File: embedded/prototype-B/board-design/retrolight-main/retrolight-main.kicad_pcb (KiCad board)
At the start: 2 copper layers, 57 x 19 mm, 31 parts, among them J1 Conn_02x03_Odd_Even, U1 TLC59108xPW

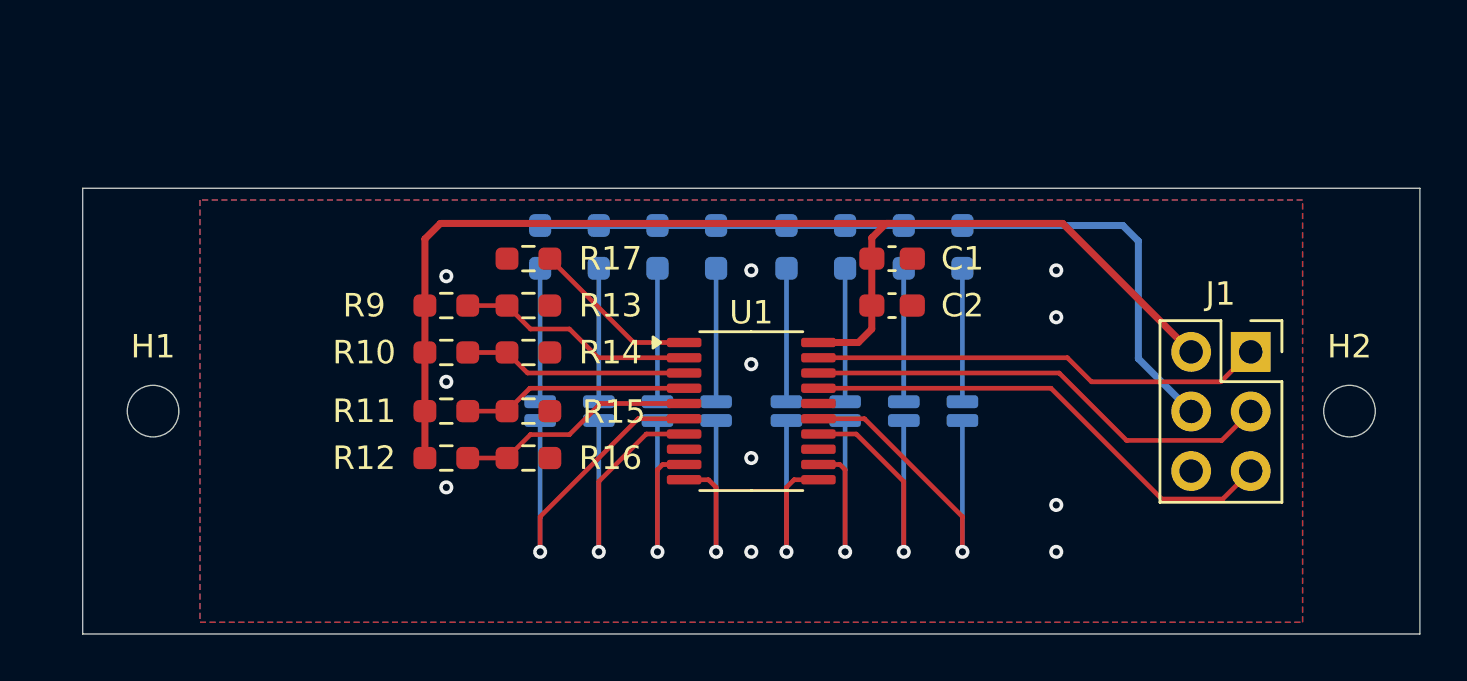
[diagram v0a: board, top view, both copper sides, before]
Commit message: [Light] Rework
Refactored light module design to match the newest changes for the
central unit.

Signed-off-by: Nicolae-Andrei Prodan <vasilenicolaeandrei@gmail.com>
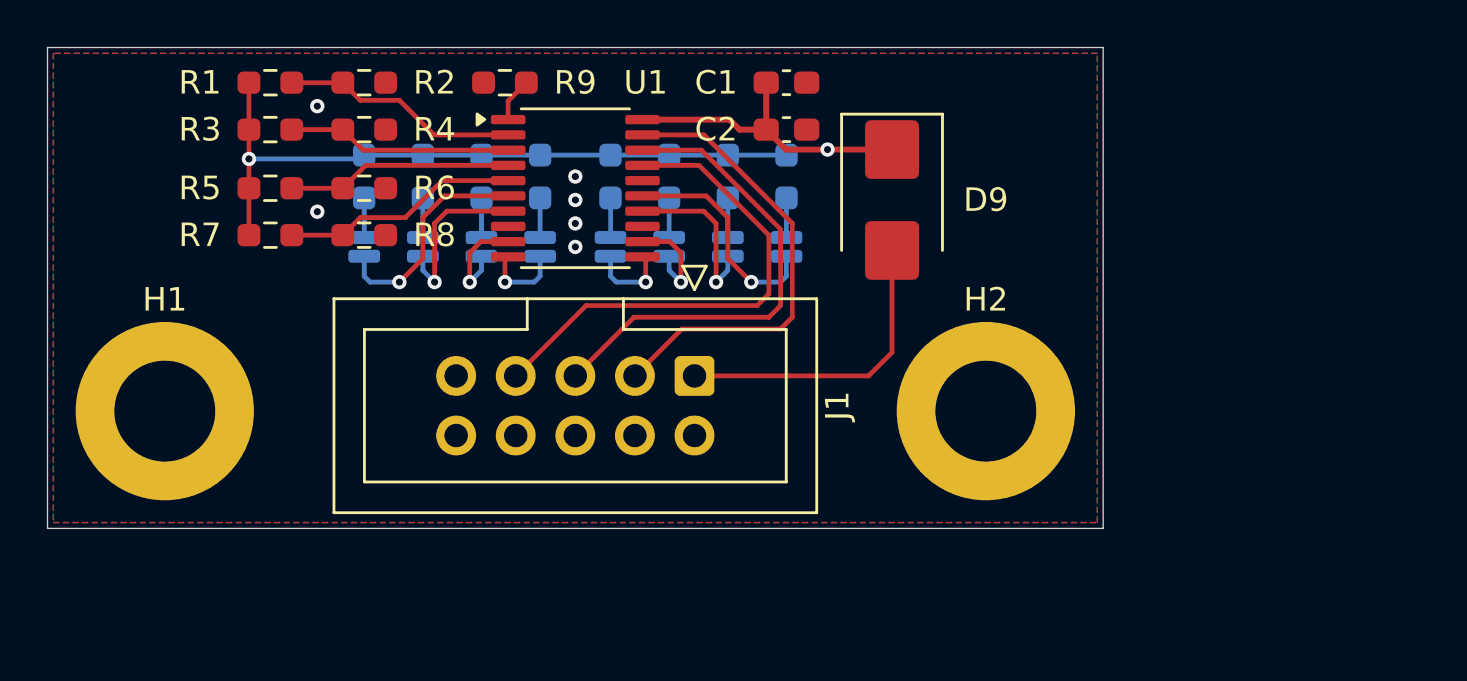
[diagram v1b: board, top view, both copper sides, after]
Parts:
- added D9: MBRS130LT3G, Diode_SMD:D_SMB, F.Cu at (156.0, 91.0)
- H1, H2: value MountingHole -> MountingHole_Pad; footprint MountingHole:MountingHole_2.2mm_M2_ISO7380 -> MountingHole:MountingHole_4.3mm_M4_ISO7380_Pad
- J1: value Conn_02x03_Odd_Even -> Conn_02x05_Odd_Even; footprint Connector_PinSocket_2.54mm:PinSocket_2x03_P2.54mm_Vertical -> Connector_IDC:IDC-Header_2x05_P2.54mm_Vertical
- R1, R3, R5, R7: value 0R/R0603 -> 10K/R0603(NC); moved to F.Cu
- R10, R11, R12: value 10K/R0603(NC) -> 0R/R0603; moved to B.Cu
- R13, R14, R15, R16: moved to B.Cu
- R17: value 375R/R0603 -> 0R/R0603; moved to B.Cu
- R2, R4, R6, R8: moved to F.Cu
- R9: value 10K/R0603(NC) -> 375R/R0603
- moved R7 27.0 mm to (129.5, 92.5), turned to 180 degrees
- moved R8 25.5 mm to (133.5, 92.5), turned to 0 degrees
- moved J1 23.7 mm to (147.6, 98.5), turned to -90 degrees
- moved R5 22.1 mm to (129.5, 90.5), turned to 180 degrees
- moved R6 20.7 mm to (133.5, 90.5), turned to 0 degrees
- moved R3 17.2 mm to (129.5, 88.0), turned to 180 degrees
- moved R4 15.8 mm to (133.5, 88.0), turned to 0 degrees
- moved H2 15.5 mm to (160.0, 100.0)
- moved R16 14.7 mm to (149.0, 90.0), turned to 90 degrees
- moved R1 13.5 mm to (129.5, 86.0), turned to 180 degrees
- moved R2 12.2 mm to (133.5, 86.0), turned to 0 degrees
- moved U1 12.1 mm to (142.5, 90.5)
- moved R12 12.1 mm to (138.5, 90.0), turned to 90 degrees
- moved R15 11.7 mm to (146.5, 90.0), turned to 90 degrees
- moved R17 11.5 mm to (151.5, 90.0), turned to 90 degrees
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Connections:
- J1 pad 1: /SDA -> Net-(D9-A)
- J1 pad 2: VCC -> unconnected-(J1-Pin_2-Pad2)
- J1 pad 3: /SCL -> /SDA
- J1 pad 4: VLED -> unconnected-(J1-Pin_4-Pad4)
- J1 pad 5: /~{RESET} -> /SCL
- J1 pad 6: GND -> unconnected-(J1-Pin_6-Pad6)
- R1 pad 1: Net-(D1-A) -> Net-(U1-A0)
- R1 pad 2: VLED -> VCC
- R10 pad 1: Net-(U1-A1) -> Net-(D1-A)
- R11 pad 1: Net-(U1-A2) -> Net-(D2-A)
- R12 pad 1: Net-(U1-A3) -> Net-(D3-A)
- R13 pad 1: Net-(U1-A0) -> Net-(D4-A)
- R13 pad 2: GND -> VCC
- R14 pad 1: Net-(U1-A1) -> Net-(D5-A)
- R14 pad 2: GND -> VCC
- R15 pad 1: Net-(U1-A2) -> Net-(D6-A)
- R15 pad 2: GND -> VCC
- R16 pad 1: Net-(U1-A3) -> Net-(D7-A)
- R16 pad 2: GND -> VCC
- R17 pad 1: Net-(U1-REXT) -> Net-(D8-A)
- R17 pad 2: GND -> VCC
- R2 pad 1: Net-(D2-A) -> Net-(U1-A0)
- R2 pad 2: VLED -> GND
- R3 pad 1: Net-(D3-A) -> Net-(U1-A1)
- R3 pad 2: VLED -> VCC
- R4 pad 1: Net-(D4-A) -> Net-(U1-A1)
- R4 pad 2: VLED -> GND
- R5 pad 1: Net-(D5-A) -> Net-(U1-A2)
- R5 pad 2: VLED -> VCC
- R6 pad 1: Net-(D6-A) -> Net-(U1-A2)
- R6 pad 2: VLED -> GND
- R7 pad 1: Net-(D7-A) -> Net-(U1-A3)
- R7 pad 2: VLED -> VCC
- R8 pad 1: Net-(D8-A) -> Net-(U1-A3)
- R8 pad 2: VLED -> GND
- R9 pad 1: Net-(U1-A0) -> Net-(U1-REXT)
- R9 pad 2: VCC -> GND
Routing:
- net VLED: track 34.0 -> 0.00 mm
- net Net-(D9-A): track 0.00 -> 13.2 mm
- net VCC: track 52.1 -> 44.5 mm, vias 0 -> 2
- net Net-(D5-K): track 9.85 -> 3.59 mm
- net Net-(D4-K): track 9.85 -> 3.59 mm
- net Net-(D6-K): track 10.3 -> 4.39 mm
- net Net-(D3-K): track 10.3 -> 4.39 mm
- net Net-(D7-K): track 13.1 -> 7.16 mm
- net Net-(D2-K): track 13.1 -> 7.16 mm
- net Net-(D8-K): track 15.0 -> 9.64 mm
- net Net-(D1-K): track 15.0 -> 9.64 mm
- net Net-(U1-REXT): track 7.21 -> 1.90 mm
- net Net-(D8-A): track 5.69 -> 1.69 mm
- net Net-(D7-A): track 5.69 -> 1.69 mm
- net Net-(D6-A): track 5.69 -> 1.69 mm
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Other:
- board size 57 x 19 mm -> 45 x 20.5 mm
